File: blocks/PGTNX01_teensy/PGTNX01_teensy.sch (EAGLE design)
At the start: 43 parts, among them IC1 7805L

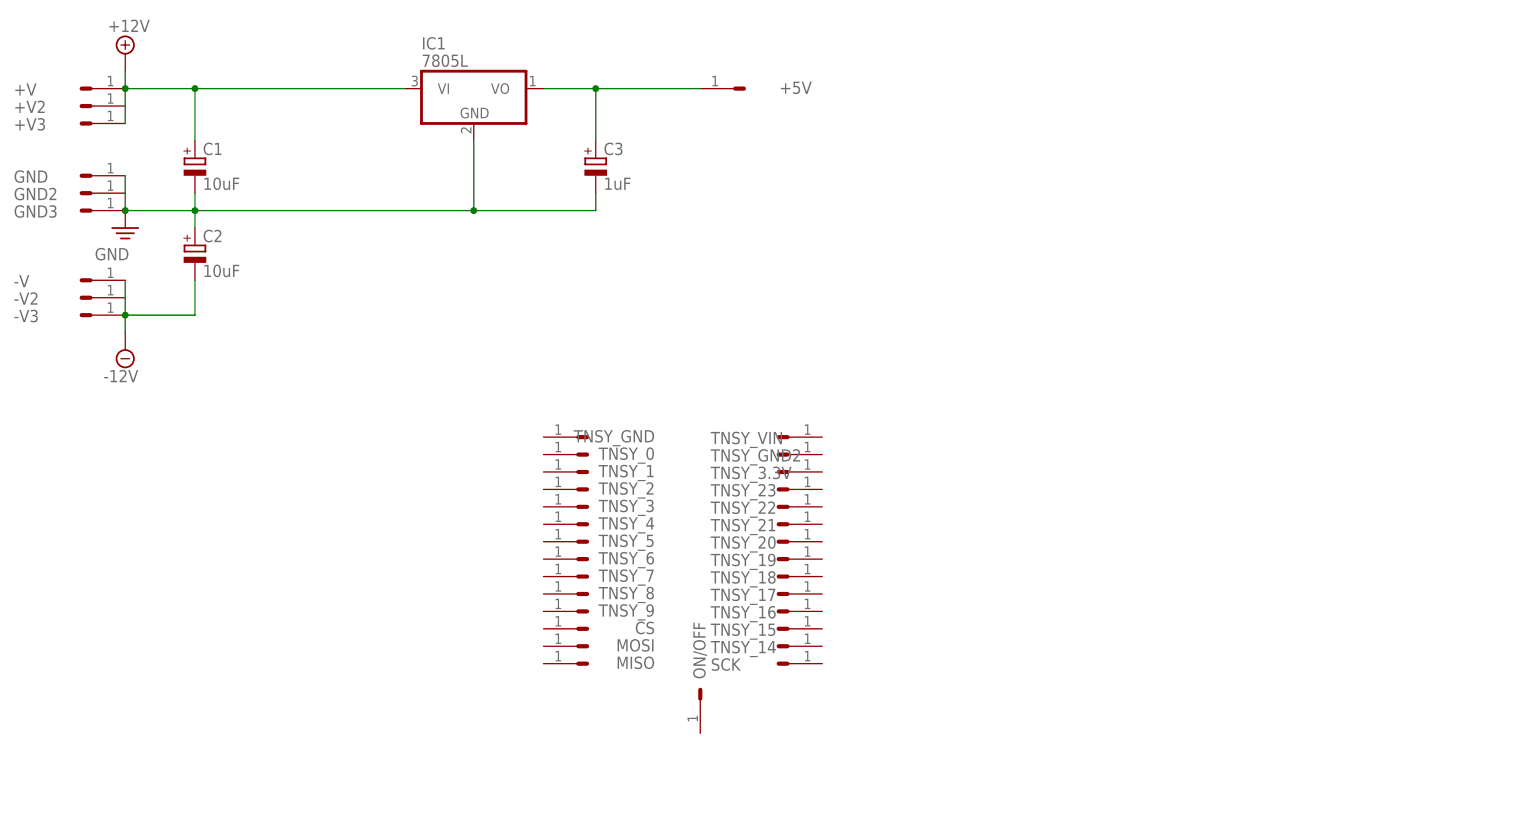
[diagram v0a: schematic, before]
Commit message: Committed a load of changes
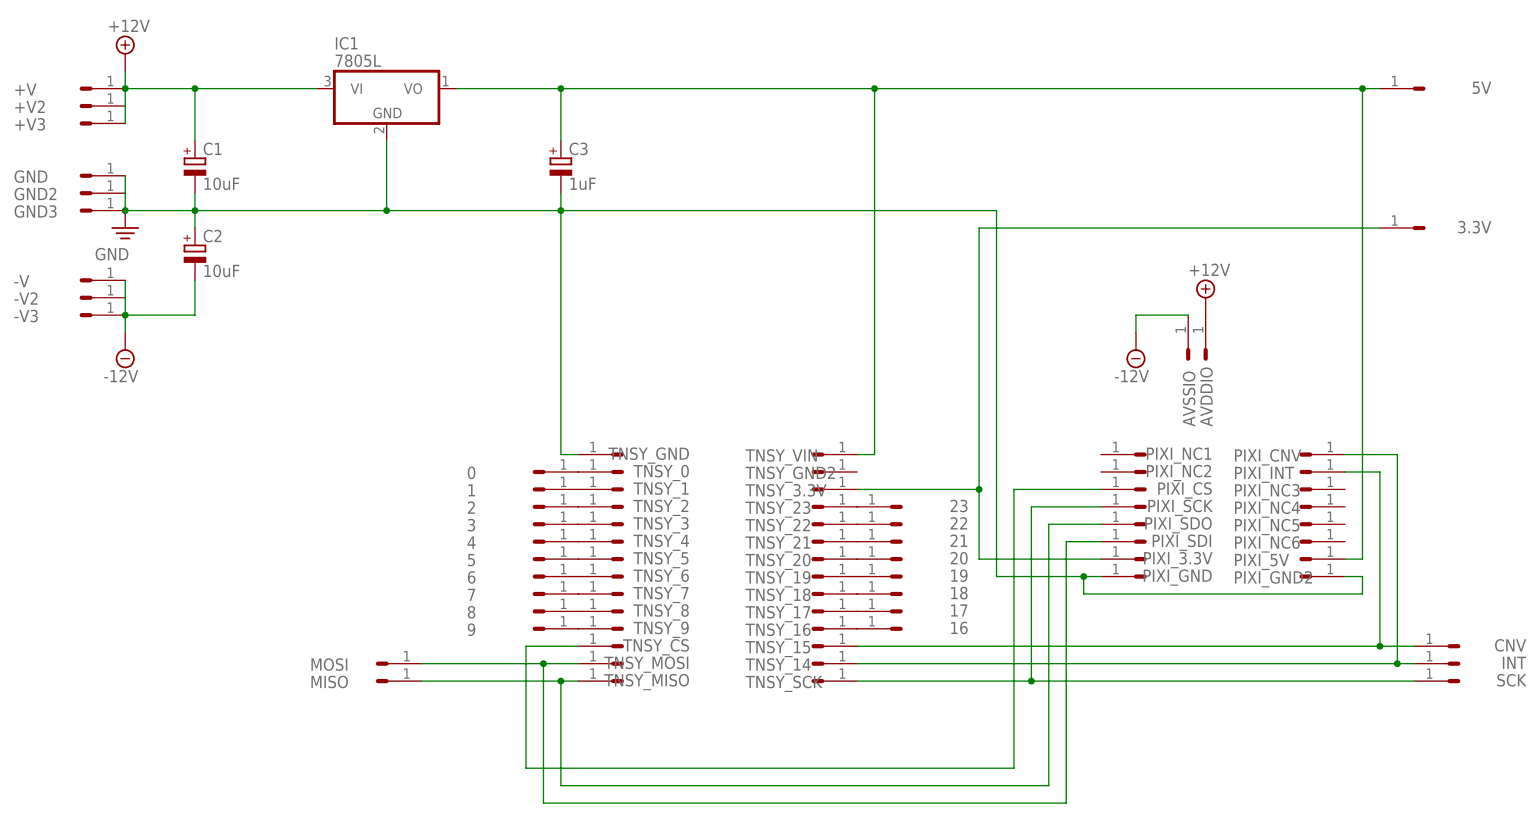
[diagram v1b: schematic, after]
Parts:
- removed +5V, ON/OFF: HEADER/MALE/01, connectors:HEADER/MALE/01
- added 0, 1, 16, 17, 18, 19, 2, 20, 21, 22, 23, 3, 3.3V, 4, 5, 5V, 6, 7, 8, AVDDIO, AVSSIO, CNV, INT, PIXI_3.3V, PIXI_5V, PIXI_CNV, PIXI_CS, PIXI_GND, PIXI_GND2, PIXI_INT, PIXI_NC1, PIXI_NC2, PIXI_NC3, PIXI_NC4, PIXI_NC5, PIXI_NC6, PIXI_SCK, PIXI_SDI, PIXI_SDO, TNSY_CS, TNSY_MISO, TNSY_MOSI, TNSY_SCK: HEADER/MALE/01, connectors:HEADER/MALE/01
- renumbered CS to 9
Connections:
- new net N$10: CNV.3, PIXI_INT.3, TNSY_15.3
- new net N$11: 18.3, TNSY_18.3
- new net N$12: 19.3, TNSY_19.3
- new net N$13: 20.3, TNSY_20.3
- new net N$14: 21.3, TNSY_21.3
- new net N$15: 22.3, TNSY_22.3
- new net N$16: 23.3, TNSY_23.3
- new net N$17: 0.3, TNSY_0.3
- new net N$18: 1.3, TNSY_1.3
- new net N$19: 2.3, TNSY_2.3
- new net N$2: 17.3, TNSY_17.3
- new net N$20: 3.3, TNSY_3.3
- new net N$21: 4.3, TNSY_4.3
- new net N$22: 5.3, TNSY_5.3
- new net N$23: 6.3, TNSY_6.3
- new net N$24: 7.3, TNSY_7.3
- new net N$25: 8.3, TNSY_8.3
- new net N$26: 9.3, TNSY_9.3
- new net N$3: 3.3V.3, PIXI_3.3V.3, TNSY_3.3V.3
- new net N$4: 16.3, TNSY_16.3
- new net N$5: MOSI.3, PIXI_SDI.3, TNSY_MOSI.3
- new net N$6: MISO.3, PIXI_SDO.3, TNSY_MISO.3
- new net N$7: PIXI_SCK.3, SCK.3, TNSY_SCK.3
- new net N$8: PIXI_CS.3, TNSY_CS.3
- new net N$9: INT.3, PIXI_CNV.3, TNSY_14.3
- net +12V: now also AVDDIO.3
- net -12V: now also AVSSIO.3
- net GND: now also PIXI_GND.3, PIXI_GND2.3, TNSY_GND.3
- net N$1: now also 5V.3, PIXI_5V.3, TNSY_VIN.3; no longer +5V.3
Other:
- moved on the sheet: C3, IC1, MISO, MOSI, SCK, TNSY_0, TNSY_1, TNSY_14, TNSY_15, TNSY_16, TNSY_17, TNSY_18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
